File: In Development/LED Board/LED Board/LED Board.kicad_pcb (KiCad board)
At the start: 2 copper layers, 33.5 x 33.5 mm, 13 parts, among them J1 Screw_Terminal_01x03, U1 AL5802

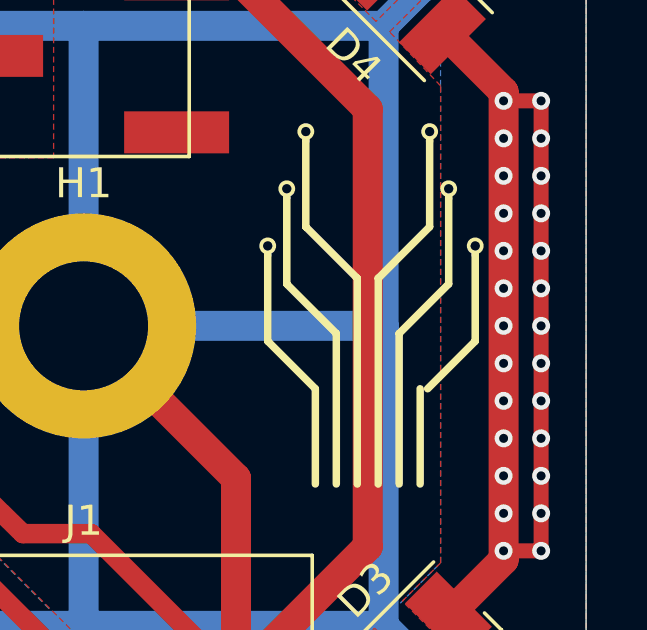
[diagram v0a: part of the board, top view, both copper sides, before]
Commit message: prep for ordering
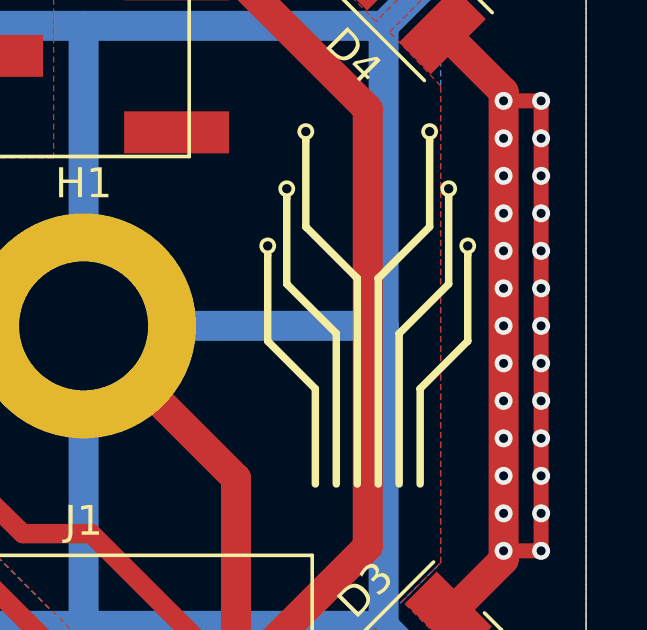
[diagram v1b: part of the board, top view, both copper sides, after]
